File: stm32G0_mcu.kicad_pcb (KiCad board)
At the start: 4 copper layers, 80 x 50 mm, 44 parts, among them J1 Conn_01x04_Pin, J2 Conn_01x06_Pin, J3 Conn_01x04_Pin, SW1 SW_Nidec_CAS-120A1, SW2 SW_Push, U1 STM32G0B0KETx, U7 MCP2200-I-SO, X1 12M

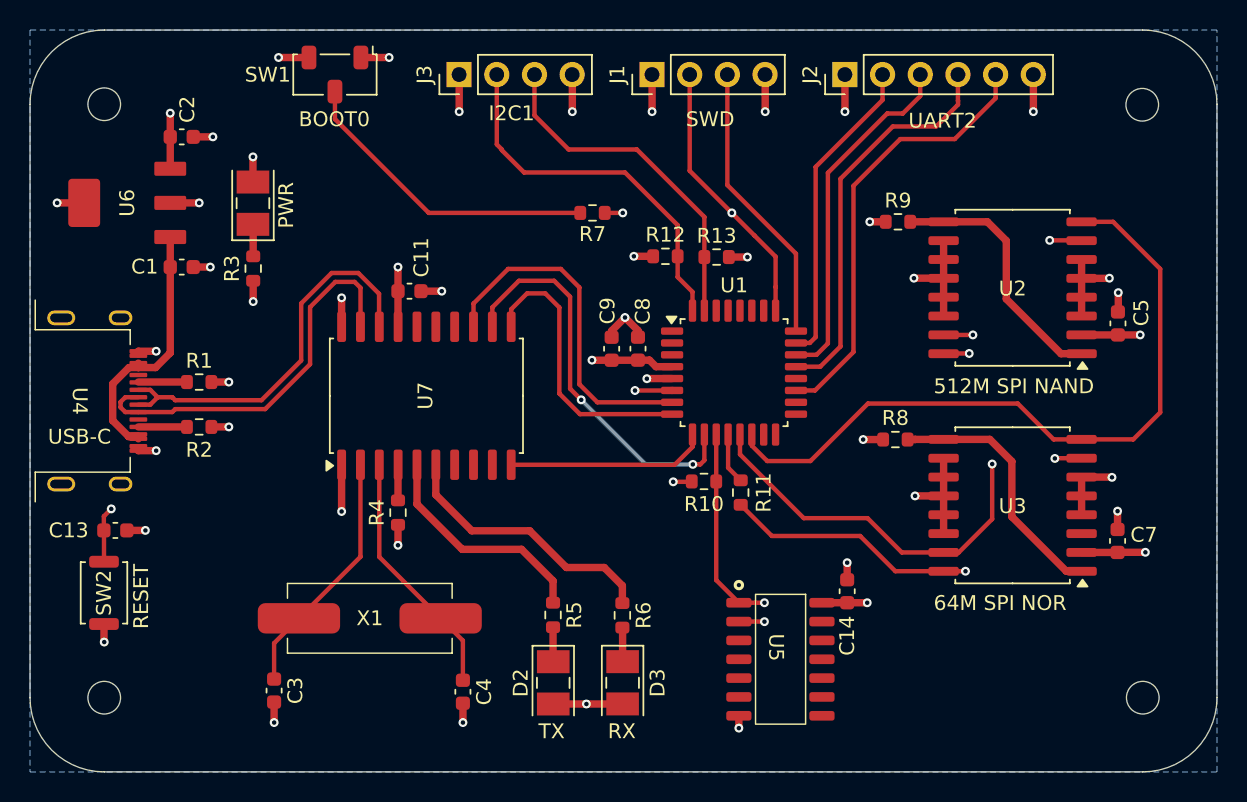
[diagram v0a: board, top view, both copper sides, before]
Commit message: asdfsa
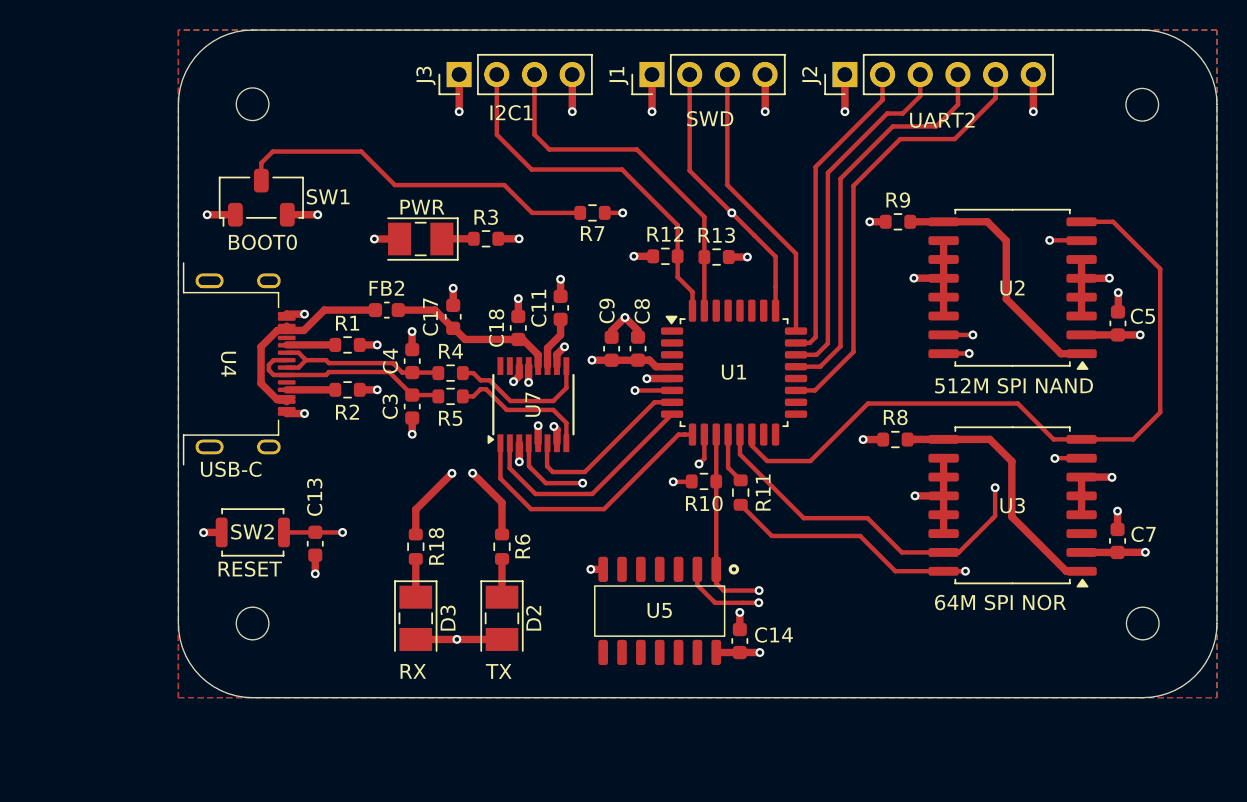
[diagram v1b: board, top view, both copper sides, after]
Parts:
- removed C1: 1u, Capacitor_SMD:C_0603_1608Metric
- removed C2: 10u, Capacitor_SMD:C_0603_1608Metric
- removed U6: ~, custom:TPS7B8333QDCYRQ1
- removed X1: 12M, custom:73-XT49M1200-S
- added C17: 100n, Capacitor_SMD:C_0603_1608Metric, F.Cu at (118.5, 99.3)
- added C18: 4u7, Capacitor_SMD:C_0603_1608Metric, F.Cu at (122.9, 100.1)
- added FB2: FerriteBead, Capacitor_SMD:C_0603_1608Metric, F.Cu at (114.0, 98.9)
- added R18: 270, Resistor_SMD:R_0603_1608Metric, F.Cu at (116.0, 114.8)
- C11, C3, C4: value C -> 47p
- R4: value 4k7 -> 27
- R5: value R -> 27
- R6: value R -> 270
- U7: value MCP2200-I-SO -> FT230XS; footprint Package_SO:SOIC-20W_7.5x12.8mm_P1.27mm -> Package_SO:SSOP-16_3.9x4.9mm_P0.635mm
- moved C4 22.5 mm to (115.8, 102.3), turned to 90 degrees
- moved C3 21.3 mm to (115.8, 105.4)
- moved R5 16.3 mm to (118.3, 104.7), turned to 0 degrees
- moved R3 15.8 mm to (120.7, 94.1), turned to 180 degrees
- moved D3 14.6 mm to (116.0, 119.7)
- moved C13 13.5 mm to (109.2, 114.6), turned to 90 degrees
- moved D1 11.6 mm to (116.3, 94.1), turned to 180 degrees
- moved H4 11.2 mm to (105.0, 120.0)
- moved SW2 10.8 mm to (105.0, 113.9), turned to 0 degrees
- moved R1 10.3 mm to (111.4, 101.2)
- moved R2 10.3 mm to (111.4, 104.2)
- moved U4 10.3 mm to (103.3, 102.5)
- moved C11 10.2 mm to (125.8, 98.7), turned to 90 degrees
- moved R4 10.0 mm to (118.3, 103.1), turned to 0 degrees
- moved H1 10.0 mm to (105.0, 85.0)
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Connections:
- net UART1_CTS renamed ~{UART1_CTS}
- net UART1_RTS renamed ~{UART1_RTS}
- C11 pad 1: +3.3V -> Net-(U7-~{RESET})
- C3 pad 1: /UART/OSC1 -> USB_D+
- C4 pad 1: /UART/OSC2 -> USB_D-
- R4 pad 1: +3.3V -> USB_D-
- R4 pad 2: /UART/RST -> USB_D-
- R5 pad 1: /UART/TX_LED -> USB_D+
- R5 pad 2: Net-(D2-A) -> USB_D+
- R6 pad 1: /UART/RX_LED -> /POWER_SUPPLY/TX_LED
- R6 pad 2: Net-(D3-A) -> Net-(D2-A)
- U1 pad 7: UART2_CTS -> ~{UART2_CTS}
- U1 pad 8: UART2_RTS -> ~{UART2_RTS}
- U2 pad 8: /FLASH/SPI1_MISO -> SPI1_MISO
- U3 pad 8: /FLASH/SPI1_MISO -> SPI1_MISO
- U7 pad 1: +3.3V -> UART2_TX
- U7 pad 10: UART2_TX -> +3.3V
- U7 pad 11: UART2_RTS -> Net-(U7-~{RESET})
- U7 pad 12: UART2_RX -> +5V_USB
- U7 pad 13: UART2_CTS -> GND
- U7 pad 14: unconnected-(U7-GP2-Pad14) -> /POWER_SUPPLY/RX_LED
- U7 pad 2: /UART/OSC1 -> ~{UART2_RTS}
- U7 pad 3: /UART/OSC2 -> +3.3V
- U7 pad 4: /UART/RST -> UART2_RX
- U7 pad 5: /UART/TX_LED -> GND
- U7 pad 6: /UART/RX_LED -> ~{UART2_CTS}
- U7 pad 7: unconnected-(U7-GP5-Pad7) -> /POWER_SUPPLY/TX_LED
- U7 pad 8: unconnected-(U7-GP4-Pad8) -> USB_D+
- U7 pad 9: unconnected-(U7-GP3-Pad9) -> USB_D-
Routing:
- net UART2_CTS: track 23.5 -> 0.00 mm
- net UART2_RTS: track 19.2 -> 0.00 mm
- net /UART/RX_LED: track 18.3 -> 0.00 mm
- net /UART/OSC2: track 16.9 -> 0.00 mm
- net /UART/OSC1: track 16.9 -> 0.00 mm
- net ~{UART2_RTS}: track 0.00 -> 15.6 mm
- net /UART/TX_LED: track 15.4 -> 0.00 mm
- net /POWER_SUPPLY/TX_LED: track 0.00 -> 14.7 mm, vias 0 -> 2
- net /POWER_SUPPLY/RX_LED: track 0.00 -> 14.2 mm, vias 0 -> 2
- net NRST: track 44.9 -> 31.0 mm
- net ~{UART2_CTS}: track 0.00 -> 12.1 mm
- net UART2_RX: track 26.9 -> 16.2 mm
- net +3.3V: track 46.2 -> 36.6 mm, vias 18 -> 16
- net +5V_USB: track 18.3 -> 25.8 mm
- net USB_D-: track 26.6 -> 21.8 mm
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- added copper zone on F.Cu, net GND
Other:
- board size 80 x 50 mm -> 70 x 45 mm
- board text added: "KabelitzJ STM32G0 Dev Board Rev. 1 29.10.2024"
- board text removed: "KabelitzJ STM32G0 Dev Board Rev 1 29.10.2024"
